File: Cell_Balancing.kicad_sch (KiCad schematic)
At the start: 30 parts, among them IC6 BQ7694204PFBR, J6 Conn_01x06, J7 Conn_01x04, Q10 MMBT5551LT1G

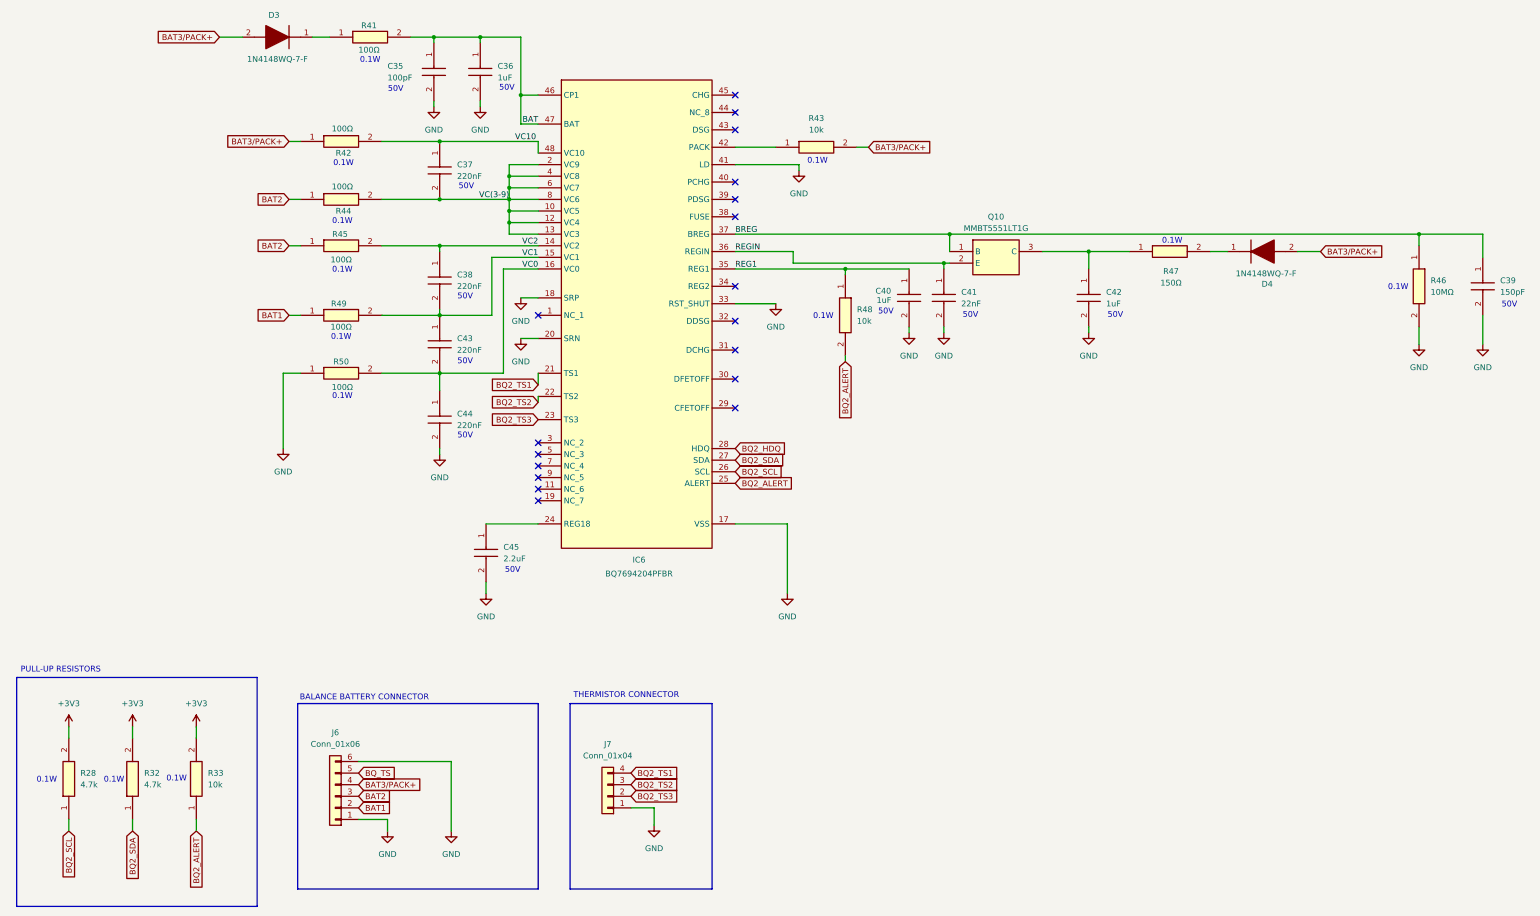
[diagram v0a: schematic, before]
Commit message: First Changes
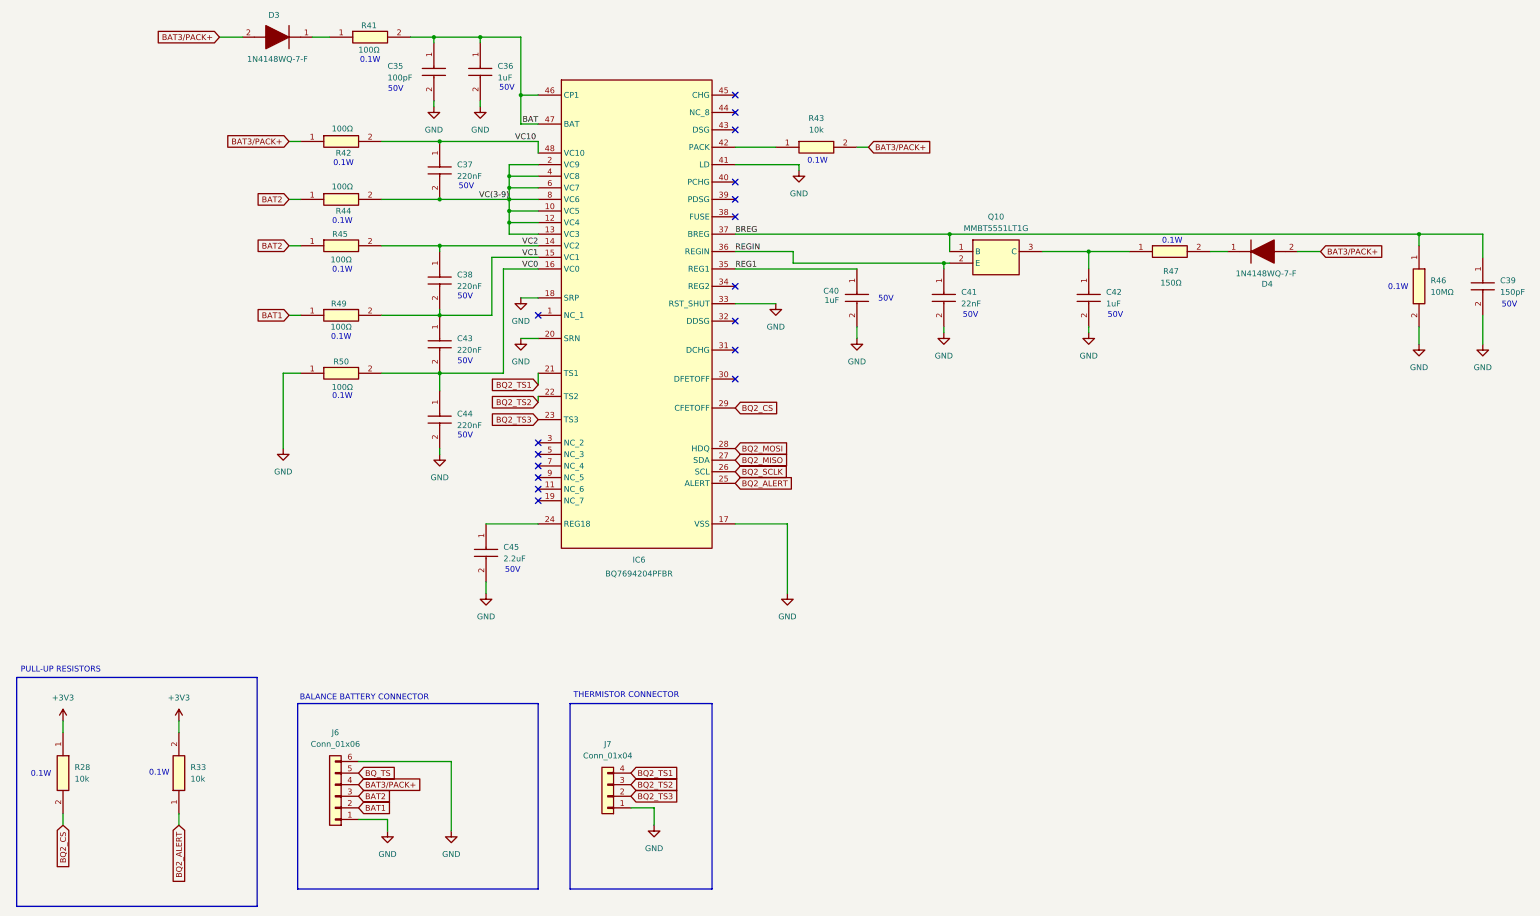
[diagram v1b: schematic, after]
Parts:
- removed R28, R32: 4.7k, RC0603FR-074K7L:RESC1608X55N, symbol RC0603FR-074K7L:RC0603FR-074K7L
- removed R48: 10k, RC0603FR-0710KL:RESC1608X55N, symbol RC0603FR-0710KL:RC0603FR-0710KL
- added R28: 10k, RC0603FR-0710KL:RESC1608X55N, symbol RC0603FR-0710KL:RC0603FR-0710KL
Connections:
- net +3V3: now also R28.1
- net BQ2_CS: now reaches IC6.29 (CFETOFF)
- net BQ2_CS: now also R28.2
- net BQ2_HDQ renamed BQ2_MOSI
- net BQ2_SCL renamed BQ2_SCLK
- net BQ2_SDA renamed BQ2_MISO
- no-connect marks 18 -> 17
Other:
- moved on the sheet: C40, R33
